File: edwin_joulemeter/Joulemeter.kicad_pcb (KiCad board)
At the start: 2 copper layers, 159.8 x 99.8 mm, 53 parts, among them J1 XT60-M, J2 22035035, J3 22035035, J4 XT60-M, U1 INA240A1PWR, U3 MCP6286T-E/OT, U4 PADS131M04QPWRQ1, U5 LTC1258CMS8-5-PBF

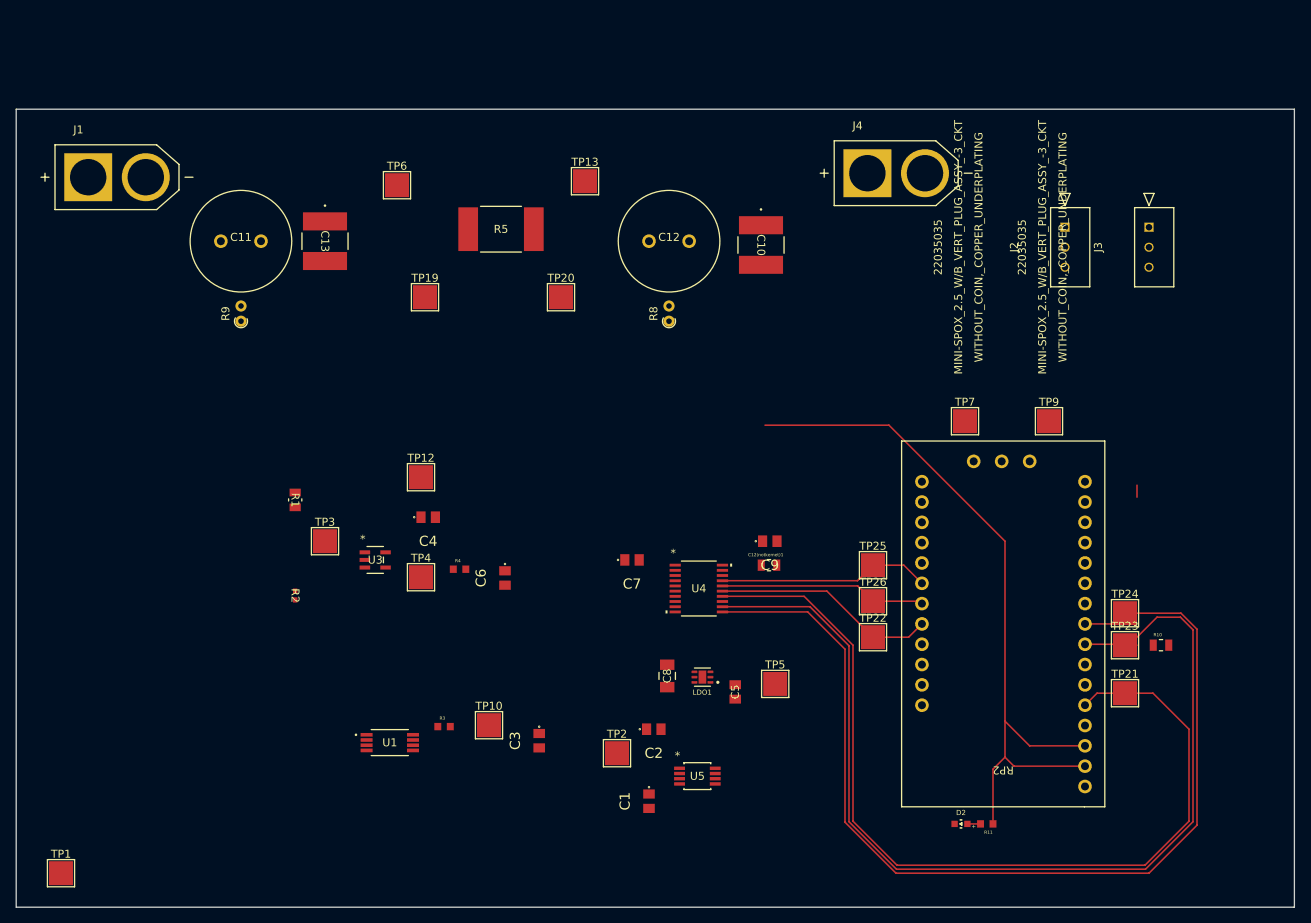
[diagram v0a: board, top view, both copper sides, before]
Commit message: updated 1/15/25
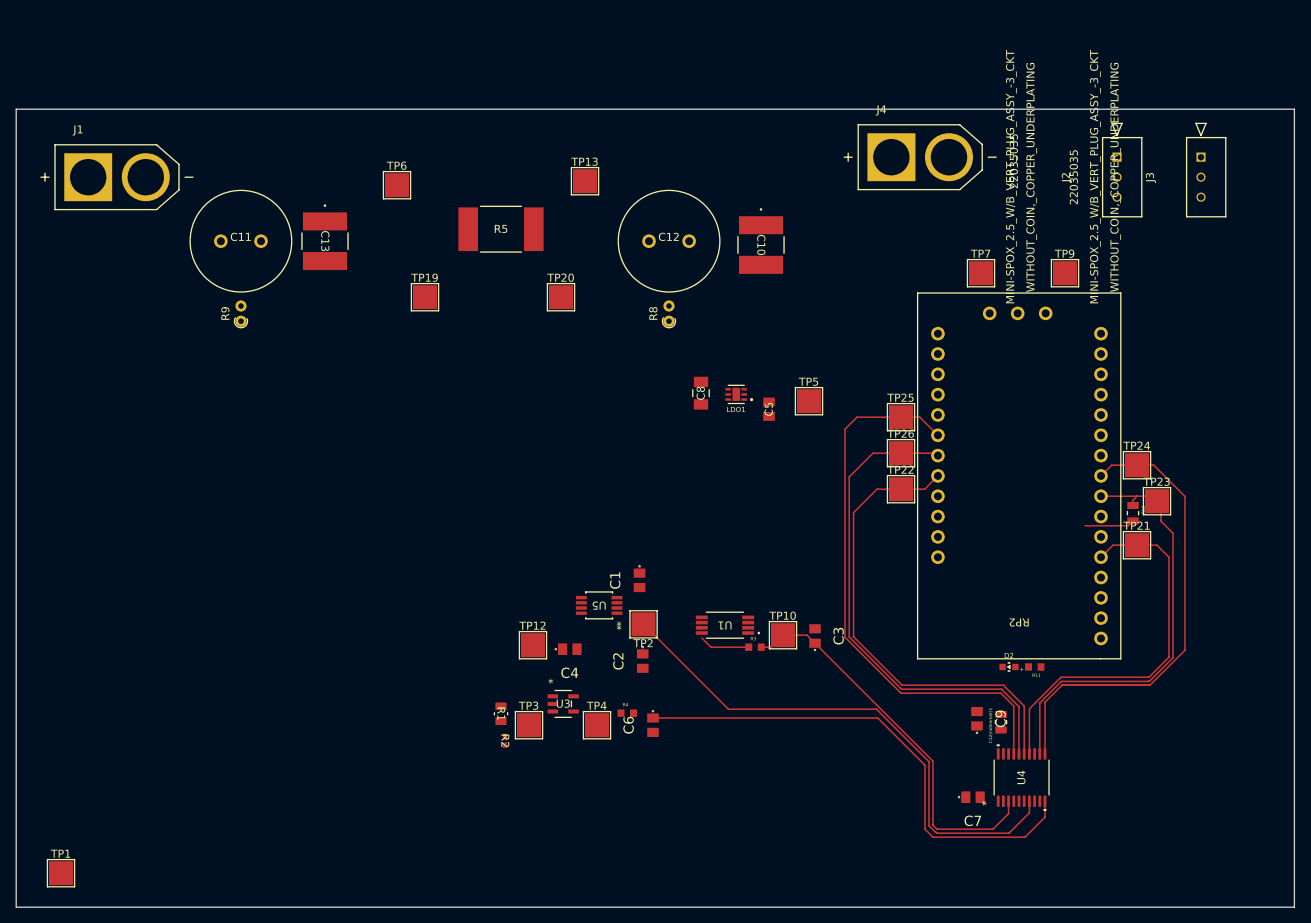
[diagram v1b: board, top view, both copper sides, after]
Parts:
- moved C7 51.9 mm to (141.0, 117.5)
- moved U4 46.8 mm to (147.1, 115.0), turned to 90 degrees
- moved U1 44.4 mm to (110.0, 96.0), turned to 180 degrees
- moved R3 40.1 mm to (113.8, 98.8)
- moved TP10 38.4 mm to (117.2, 97.2)
- moved R1 37.1 mm to (82.0, 107.1)
- moved C3 36.9 mm to (121.2, 97.3), turned to 90 degrees
- moved C5 35.6 mm to (115.5, 69.0)
- moved C8 35.6 mm to (107.0, 67.0)
- moved LDO1 35.6 mm to (111.4, 67.2)
- moved TP5 35.6 mm to (120.5, 68.0)
- moved C12(notkemet)1 35.0 mm to (144.5, 108.1), turned to 90 degrees
- moved TP3 34.3 mm to (85.5, 108.5)
- moved C9 34.1 mm to (141.5, 107.7), turned to 90 degrees
- moved R2 31.9 mm to (82.5, 110.5)
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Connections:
- U4 pad 10: unconnected-(U4-AIN3P-Pad10) -> /V_ADC
- U4 pad 5: GND -> unconnected-(U4-AIN1N-Pad5)
- U4 pad 6: /V_ADC -> unconnected-(U4-AIN1P-Pad6)
- U4 pad 9: unconnected-(U4-AIN3N-Pad9) -> GND
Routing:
- net +3V3: track 93.7 -> 6.25 mm
- net /CS: track 128.9 -> 54.7 mm
- net /SCK: track 114.4 -> 48.0 mm
- net +1V65: track 0.00 -> 66.2 mm
- net /V_ADC: track 0.00 -> 62.9 mm
- net /GPIO_RESET: track 129.4 -> 71.5 mm
- net /I_ADC: track 0.00 -> 48.6 mm
- net /GPIO_CLKIN: track 26.7 -> 69.8 mm
- net /MOSI: track 25.8 -> 63.2 mm
- net /MISO: track 28.0 -> 58.9 mm
- net Net-(U1-OUT): track 0.00 -> 6.84 mm
- net Net-(D2-Pad2): track 1.64 -> 0.00 mm
